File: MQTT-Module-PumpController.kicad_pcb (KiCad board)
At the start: 4 copper layers, 44 x 55.9 mm, 36 parts, among them IC801 LM5060MMX_NOPB, J301 A2541WV-10P, J302 A2541WV-10P, J303 1715721, J304 A2541HWV-3P, Q801 60V 38A, U201 ATtiny1614-SS

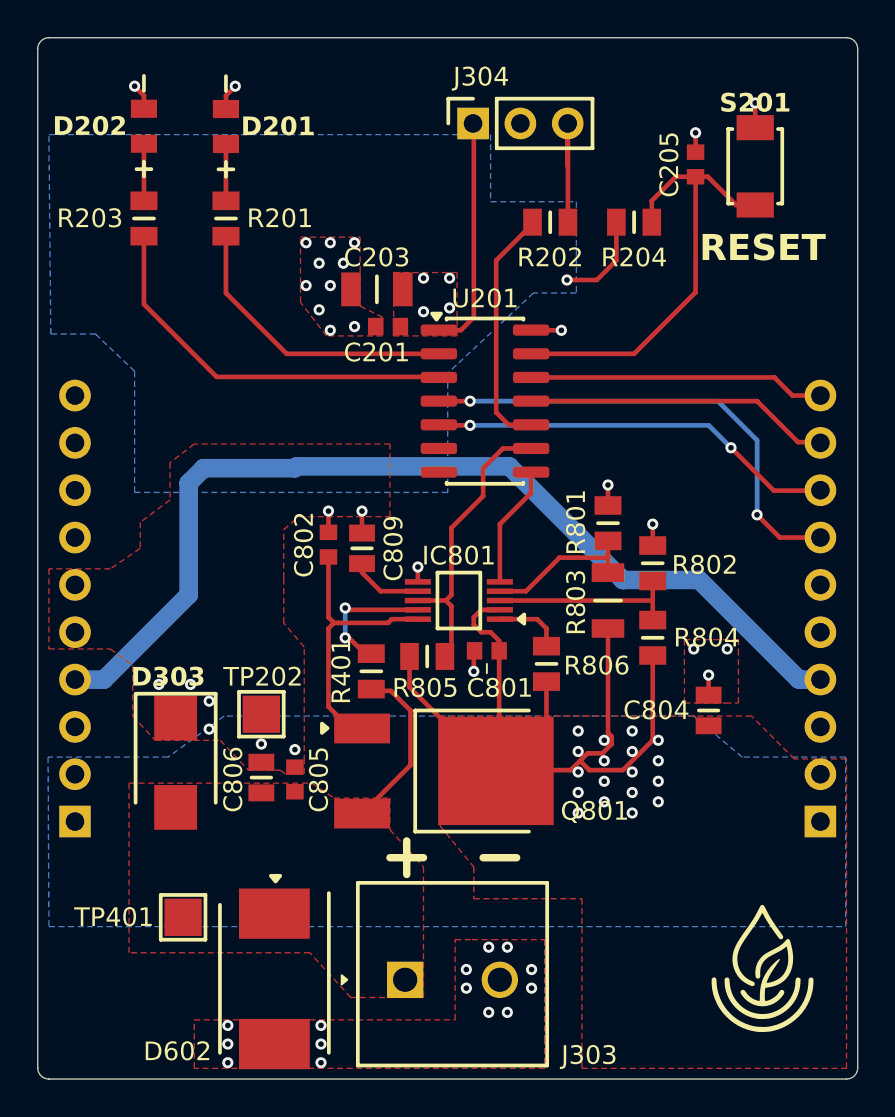
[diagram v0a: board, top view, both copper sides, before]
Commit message: Finalised silkscreen. Generated outputs.
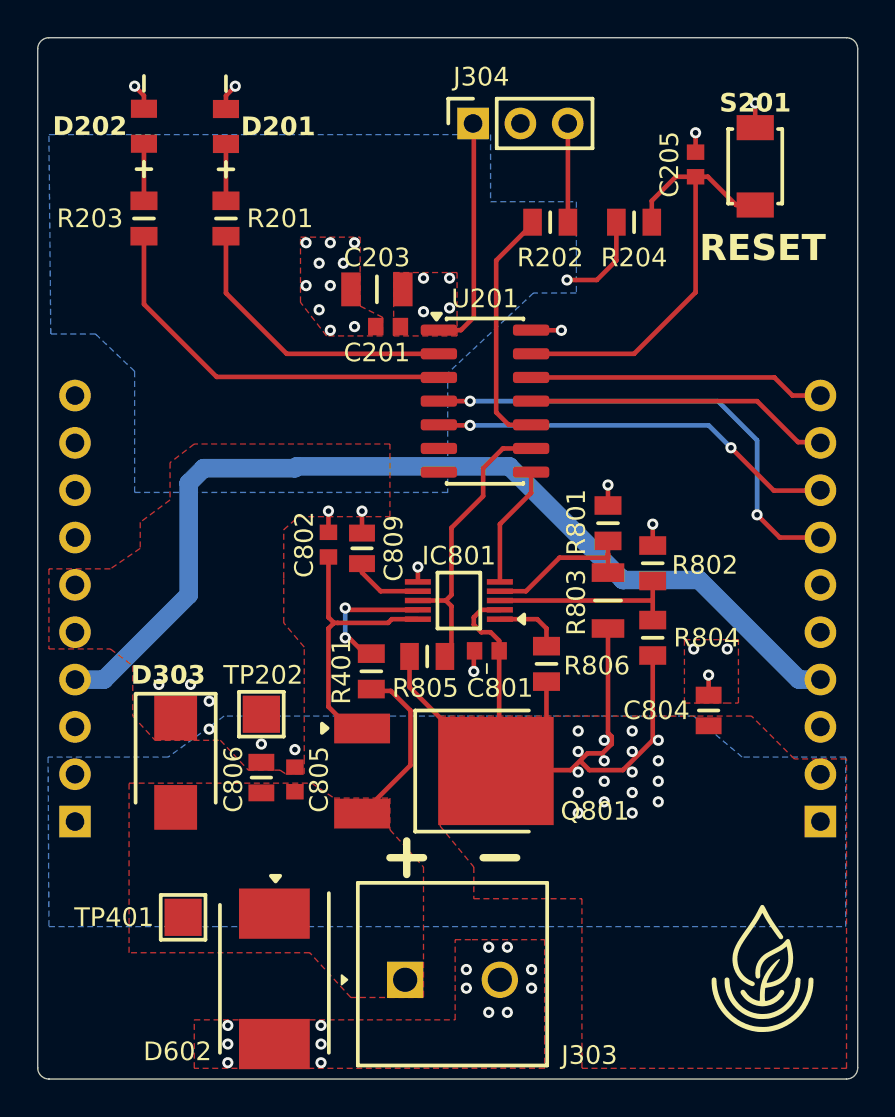
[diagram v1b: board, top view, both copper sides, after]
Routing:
- net /Controller/UDPI_C: track 7.60 -> 5.30 mm
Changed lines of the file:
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@@
 		(tags "Diode SMB (DO-214AA)")
 		(property "Reference" "D303"
-			(at -4.6 0.4 180)
+			(at -4.7 0.4 180)
 			(layer "F.SilkS")
 			(effects
@@
 		(tags "test point SMD pad rectangle square")
 		(property "Reference" "TP202"
-			(at 0.1 -1.998 0)
+			(at 0.1 -2.1 0)
 			(layer "F.SilkS")
 			(effects
@@
 		(width 0.25)
 		(layer "F.Cu")
-		(net 24)
-	)
-	(segment
-		(start 146.44 72.6)
-		(end 146.44 74.9)
-		(width 0.25)
-		(layer "F.Cu")
